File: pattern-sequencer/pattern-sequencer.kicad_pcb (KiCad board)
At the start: 2 copper layers, 90.2 x 151.8 mm, 64 parts, among them J1 Power, J10 Conn_01x03_Socket, J11 Conn_01x03_Socket, J12 Conn_01x03_Socket, J13 Conn_01x03_Socket, J14 Conn_01x03_Socket, J2 Power, J3 Power, J4 External Clock, J5 Conn_01x03_Socket, J6 Out 1, J7 Out 2, J8 Out 3, J9 Out 4, SW1 IN 1, SW2 IN 2, SW3 IN 3, SW4 IN 4, SW5 CLEAR, SW6 External Clock Select

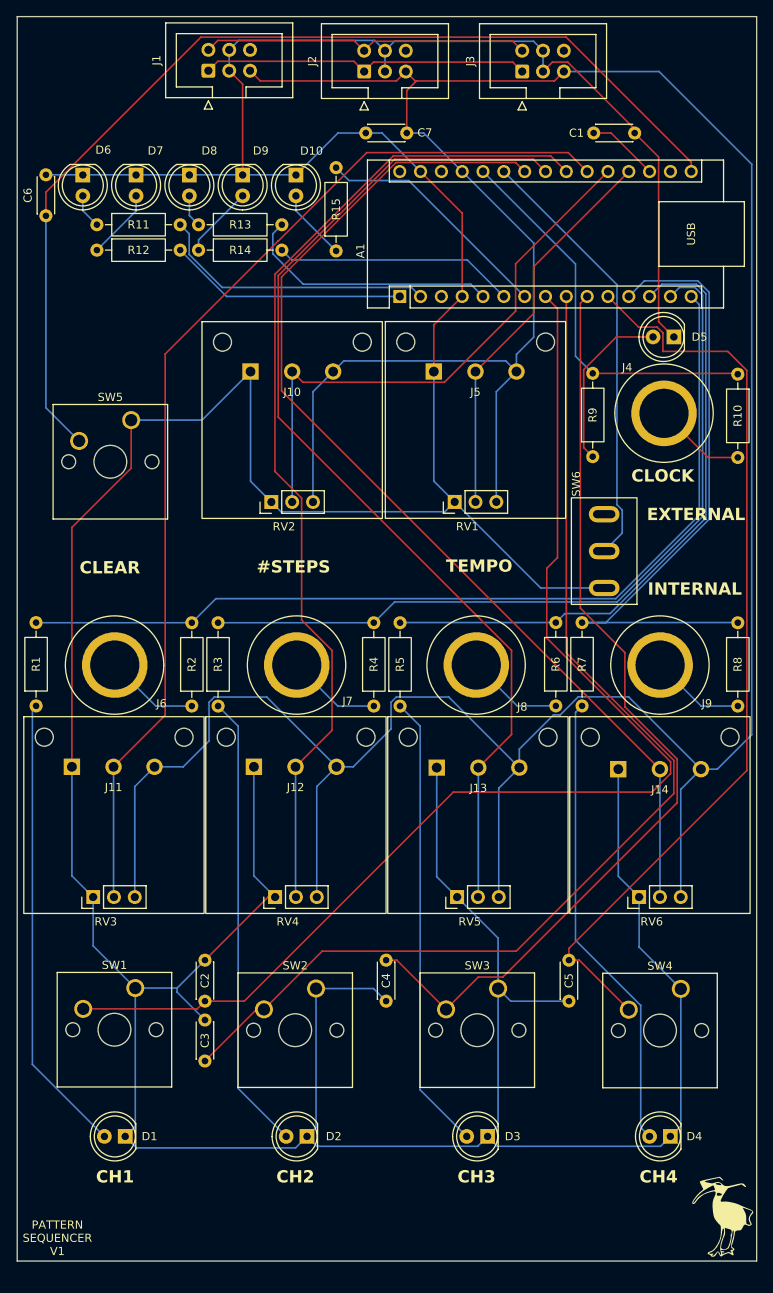
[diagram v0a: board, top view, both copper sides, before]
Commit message: Update pattern sequencer
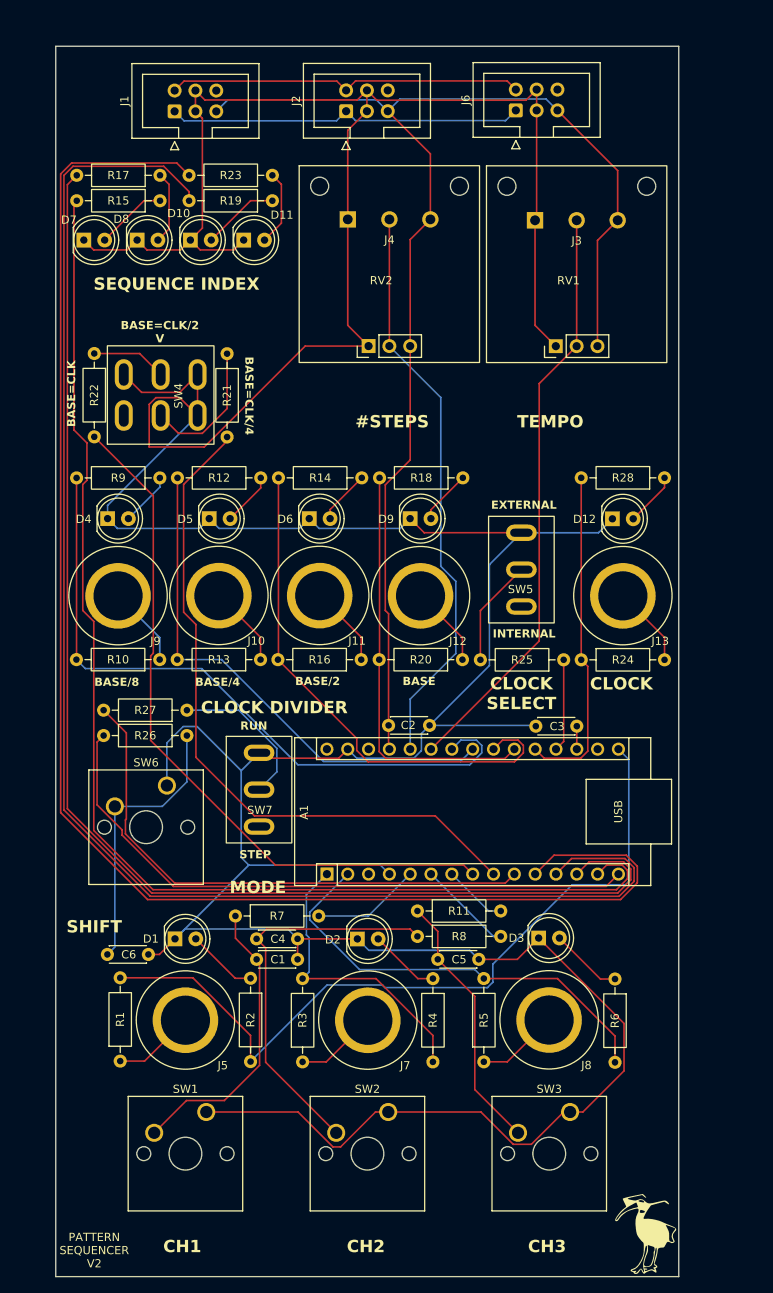
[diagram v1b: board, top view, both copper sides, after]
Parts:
- removed C7: 100nf, Capacitor_THT:C_Disc_D4.3mm_W1.9mm_P5.00mm
- removed J14: Conn_01x03_Socket, modular2:pot
- removed RV3: 100K - Len 1, modular2:pot-socket
- removed RV4: 100K - Len 2, modular2:pot-socket
- removed RV5: 100K - Len 3, modular2:pot-socket
- removed RV6: 100K - Len 4, modular2:pot-socket
- added D11: LED (Red), LED_THT:LED_D5.0mm, F.Cu at (88.8, 48.9)
- added D12: LED (Red), LED_THT:LED_D5.0mm, F.Cu at (133.8, 82.9)
- added R16: 1K, Resistor_THT:R_Axial_DIN0207_L6.3mm_D2.5mm_P10.16mm_Horizontal, F.Cu at (103.2, 100.0)
- added R17: 1K, Resistor_THT:R_Axial_DIN0207_L6.3mm_D2.5mm_P10.16mm_Horizontal, F.Cu at (78.6, 41.0)
- added R18: 1K, Resistor_THT:R_Axial_DIN0207_L6.3mm_D2.5mm_P10.16mm_Horizontal, F.Cu at (115.6, 77.9)
- added R19: 1K, Resistor_THT:R_Axial_DIN0207_L6.3mm_D2.5mm_P10.16mm_Horizontal, F.Cu at (92.3, 44.1)
- added R20: 1K, Resistor_THT:R_Axial_DIN0207_L6.3mm_D2.5mm_P10.16mm_Horizontal, F.Cu at (115.5, 100.0)
- added R21: 1K, Resistor_THT:R_Axial_DIN0207_L6.3mm_D2.5mm_P10.16mm_Horizontal, F.Cu at (86.8, 62.7)
- added R22: 1K, Resistor_THT:R_Axial_DIN0207_L6.3mm_D2.5mm_P10.16mm_Horizontal, F.Cu at (70.6, 62.7)
- added R23: 1K, Resistor_THT:R_Axial_DIN0207_L6.3mm_D2.5mm_P10.16mm_Horizontal, F.Cu at (92.3, 41.0)
- added R24: 1K, Resistor_THT:R_Axial_DIN0207_L6.3mm_D2.5mm_P10.16mm_Horizontal, F.Cu at (130.0, 100.1)
- added R25: 1K, Resistor_THT:R_Axial_DIN0207_L6.3mm_D2.5mm_P10.16mm_Horizontal, F.Cu at (127.9, 100.1)
- added R26: 1K, Resistor_THT:R_Axial_DIN0207_L6.3mm_D2.5mm_P10.16mm_Horizontal, F.Cu at (81.9, 109.3)
- added R27: 1K, Resistor_THT:R_Axial_DIN0207_L6.3mm_D2.5mm_P10.16mm_Horizontal, F.Cu at (81.9, 106.2)
- added R28: 1K, Resistor_THT:R_Axial_DIN0207_L6.3mm_D2.5mm_P10.16mm_Horizontal, F.Cu at (140.2, 77.9)
- added SW7: Mode Select, modular2:switch1, F.Cu at (90.7, 115.9)
- C1: value 100nf -> 1uF
- C2, C3: value 1uF -> 100nf
- J10: value Conn_01x03_Socket -> Out 1; footprint modular2:pot -> modular2:banana-jack
- J11: value Conn_01x03_Socket -> Out 2; footprint modular2:pot -> modular2:banana-jack
- J12, J5: value Conn_01x03_Socket -> Out 3; footprint modular2:pot -> modular2:banana-jack
- J13: value Conn_01x03_Socket -> External Clock; footprint modular2:pot -> modular2:banana-jack
- J3: value Power -> Conn_01x03_Socket; footprint Connector_IDC:IDC-Header_2x03_P2.54mm_Vertical -> modular2:pot
- J4: value External Clock -> Conn_01x03_Socket; footprint modular2:banana-jack -> modular2:pot
- J6: value Out 1 -> Power; footprint modular2:banana-jack -> Connector_IDC:IDC-Header_2x03_P2.54mm_Vertical
- J8: value Out 3 -> Out 1
- J9: value Out 4 -> Out 1
- SW4: value IN 4 -> Clock Divider Base Division; footprint Button_Switch_Keyboard:SW_Cherry_MX_1.00u_PCB -> modular2:switch2
- SW5: value CLEAR -> External Clock Select; footprint Button_Switch_Keyboard:SW_Cherry_MX_1.00u_PCB -> modular2:switch1
- SW6: value External Clock Select -> SHIFT; footprint modular2:switch1 -> Button_Switch_Keyboard:SW_Cherry_MX_1.00u_PCB
- moved F1 154.8 mm to (135.2, 168.1)
- moved F3 134.0 mm to (72.5, 31.8)
- moved C1 110.8 mm to (90.4, 136.6), turned to 0 degrees
- moved D4 101.9 mm to (72.2, 82.8), turned to 0 degrees
- moved SW4 96.3 mm to (78.7, 67.8), turned to 90 degrees
- moved R11 92.4 mm to (110.0, 130.7)
- moved C6 90.4 mm to (72.2, 136.0), turned to 0 degrees
- moved J5 83.9 mm to (81.7, 144.0)
- moved J6 83.5 mm to (122.0, 33.0)
- moved R10 78.6 mm to (78.6, 100.0), turned to 180 degrees
- moved F4 71.8 mm to (72.6, 168.1)
- moved A1 71.0 mm to (99.0, 126.2)
- moved J9 66.6 mm to (73.5, 92.2), turned to 0 degrees
- moved D5 60.9 mm to (84.6, 82.8), turned to 0 degrees
- moved SW6 60.5 mm to (79.5, 115.4), turned to 0 degrees
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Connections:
- C1 pad 1: GND -> Net-(C1-Pad1)
- C1 pad 2: Net-(A1-AREF) -> GND
- C2 pad 1: Net-(A1-D5) -> GND
- C2 pad 2: GND -> 5V
- C3 pad 1: Net-(A1-D6) -> GND
- C3 pad 2: GND -> Net-(A1-AREF)
- C4 pad 1: Net-(A1-D7) -> Net-(C4-Pad1)
- C5 pad 1: Net-(A1-D8) -> Net-(C5-Pad1)
- C6 pad 1: Net-(A1-D13) -> Net-(C6-Pad1)
- J10 pad 1: GND -> Net-(J10-Pin_1)
- J11 pad 1: GND -> Net-(J11-Pin_1)
- J12 pad 1: GND -> Net-(J12-Pin_1)
- J13 pad 1: GND -> Net-(J13-Pin_1)
- J3 pad 1: 12V -> GND
- J3 pad 2: -12V -> Net-(A1-A6)
- J3 pad 3: GND -> 5V
- J4 pad 1: Net-(J4-Pin_1) -> GND
- J5 pad 1: GND -> Net-(J5-Pin_1)
- J6 pad 1: Net-(J6-Pin_1) -> 12V
- R1 pad 1: Net-(D1-A) -> Net-(J5-Pin_1)
- R1 pad 2: Net-(A1-D12) -> Net-(A1-D13)
- R10 pad 1: Net-(A1-A7) -> Net-(J9-Pin_1)
- R10 pad 2: Net-(J4-Pin_1) -> Net-(A1-A5)
- R11 pad 1: Net-(D6-A) -> Net-(C5-Pad1)
- R11 pad 2: Net-(A1-D0/RX) -> Net-(A1-D4)
- R12 pad 1: Net-(D7-A) -> Net-(D5-A)
- R12 pad 2: Net-(A1-D1/TX) -> Net-(A1-A4)
- R13 pad 1: Net-(D8-A) -> Net-(J10-Pin_1)
- R13 pad 2: Net-(A1-D2) -> Net-(A1-A4)
- R14 pad 1: Net-(D9-A) -> Net-(D6-A)
- R14 pad 2: Net-(A1-D3) -> Net-(A1-A3)
- R15 pad 1: Net-(D10-A) -> Net-(D7-A)
- R15 pad 2: Net-(A1-D4) -> Net-(A1-D11)
- R2 pad 1: Net-(J6-Pin_1) -> Net-(D1-A)
- R2 pad 2: Net-(A1-D12) -> Net-(A1-D13)
- R3 pad 1: Net-(D2-A) -> Net-(J7-Pin_1)
- R3 pad 2: Net-(A1-D11) -> Net-(A1-D1/TX)
- R4 pad 1: Net-(J7-Pin_1) -> Net-(D2-A)
- R4 pad 2: Net-(A1-D11) -> Net-(A1-D1/TX)
- R5 pad 1: Net-(D3-A) -> Net-(J8-Pin_1)
- R5 pad 2: Net-(A1-D10) -> Net-(A1-D0/RX)
- R6 pad 1: Net-(J8-Pin_1) -> Net-(D3-A)
- R6 pad 2: Net-(A1-D10) -> Net-(A1-D0/RX)
- R7 pad 1: Net-(D4-A) -> Net-(C1-Pad1)
- R7 pad 2: Net-(A1-D9) -> Net-(A1-D2)
- R8 pad 1: Net-(J9-Pin_1) -> Net-(C4-Pad1)
- R8 pad 2: Net-(A1-D9) -> Net-(A1-D3)
- R9 pad 1: Net-(D5-A) -> Net-(D4-A)
- R9 pad 2: Net-(A1-A7) -> Net-(A1-A5)
- RV1 pad 2: Net-(A1-A0) -> Net-(A1-A6)
- RV2 pad 2: Net-(A1-A1) -> Net-(A1-A7)
- SW1 pad 2: Net-(A1-D5) -> Net-(C1-Pad1)
- SW2 pad 2: Net-(A1-D6) -> Net-(C4-Pad1)
- SW3 pad 2: Net-(A1-D7) -> Net-(C5-Pad1)
- SW4 pad 2: Net-(A1-D8) -> Net-(SW4A-B)
- SW5 pad 1: GND -> unconnected-(SW5-C-Pad1)
- SW5 pad 2: Net-(A1-D13) -> Net-(SW5-B)
- SW6 pad 1: unconnected-(SW6-C-Pad1) -> GND
- SW6 pad 2: Net-(A1-A6) -> Net-(C6-Pad1)
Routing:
- net 5V: track 408.3 -> 159.3 mm
- net Net-(A1-D9): track 78.6 -> 182.6 mm
- net Net-(A1-D10): track 77.9 -> 160.3 mm
- net Net-(A1-A2): track 131.5 -> 50.7 mm
- net Net-(A1-D8): track 112.7 -> 186.3 mm
- net Net-(A1-A4): track 128.4 -> 64.0 mm
- net Net-(A1-D5): track 149.1 -> 86.2 mm
- net GND: track 620.0 -> 557.0 mm
- net Net-(A1-A3): track 123.0 -> 63.9 mm
- net Net-(A1-D11): track 96.2 -> 152.4 mm
- net Net-(A1-D6): track 136.8 -> 84.1 mm
- net Net-(D4-A): track 56.6 -> 6.55 mm
- net Net-(A1-D7): track 115.4 -> 66.7 mm
- net Net-(C4-Pad1): track 0.00 -> 48.2 mm
- net Net-(A1-A5): track 130.7 -> 82.8 mm
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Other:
- board size 90.2 x 151.8 mm -> 76 x 150.1 mm
- board text added: "BASE"
- board text added: "BASE/2"
- board text added: "BASE/4"
- board text added: "BASE/8"
- board text added: "BASE=CLK"
- board text added: "BASE=CLK/2 V"
- board text added: "BASE=CLK/4"
- board text added: "CLOCK DIVIDER"
- board text added: "CLOCK SELECT"
- board text added: "MODE"
- board text added: "PATTERN SEQUENCER V2"
- board text added: "RUN"
- board text added: "SEQUENCE INDEX"
- board text added: "SHIFT"
- board text added: "STEP"
- board text removed: "CH4"
- board text removed: "CLEAR"
- board text removed: "PATTERN SEQUENCER V1"
